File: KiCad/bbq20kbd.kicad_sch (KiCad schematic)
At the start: 23 parts, among them Q3 BSS138, Q4 BSS138, Q5 BSS138, Q6 BSS138, Q7 BSS138, Q8 BSS138, U7 ME6212C18M5G, U8 ME6212C28M5G, U9 BBQ20KBD

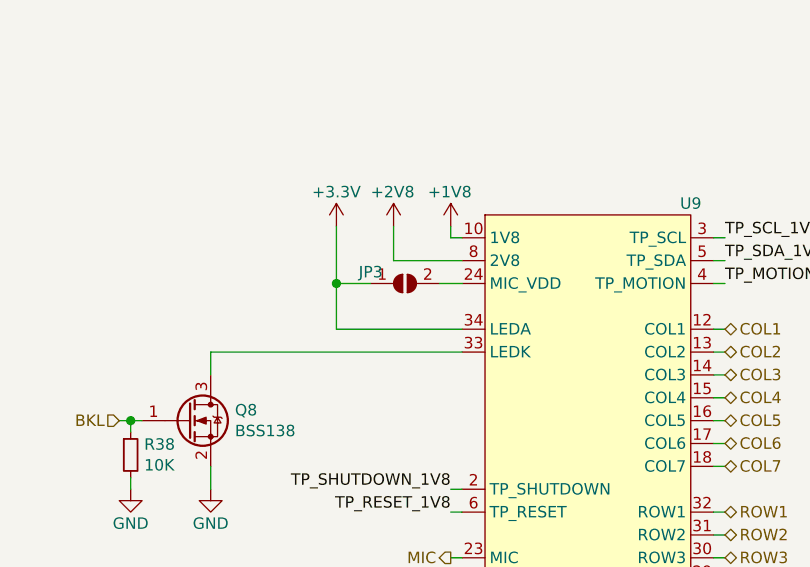
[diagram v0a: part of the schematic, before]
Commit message: update
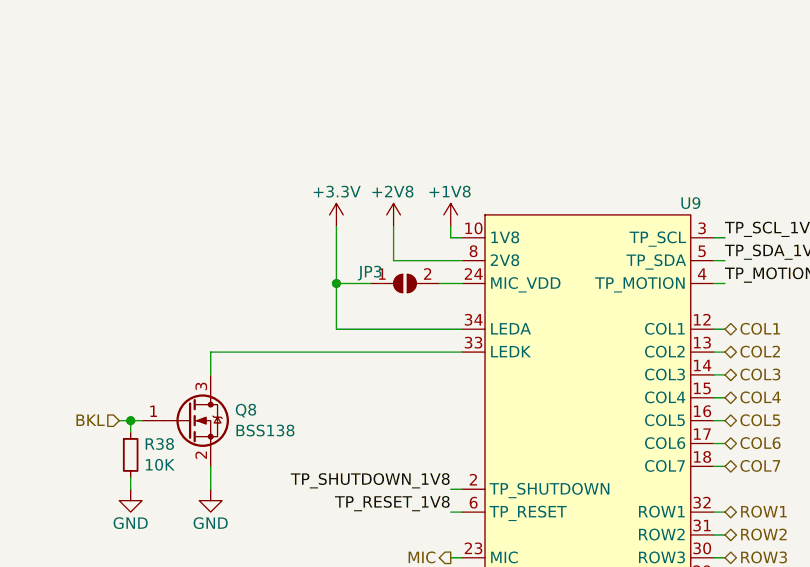
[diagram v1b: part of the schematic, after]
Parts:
- U9: footprint beepberry:BM20B(0.8)-40DS-0.4V -> beepy:BM20B(0.8)-40DS-0.4V
